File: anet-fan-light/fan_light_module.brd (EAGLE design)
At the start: 10 parts, among them X1 12V, X2 EXT-FAN, X3 Z-PROBE, X4 ANET-Z-INPUT

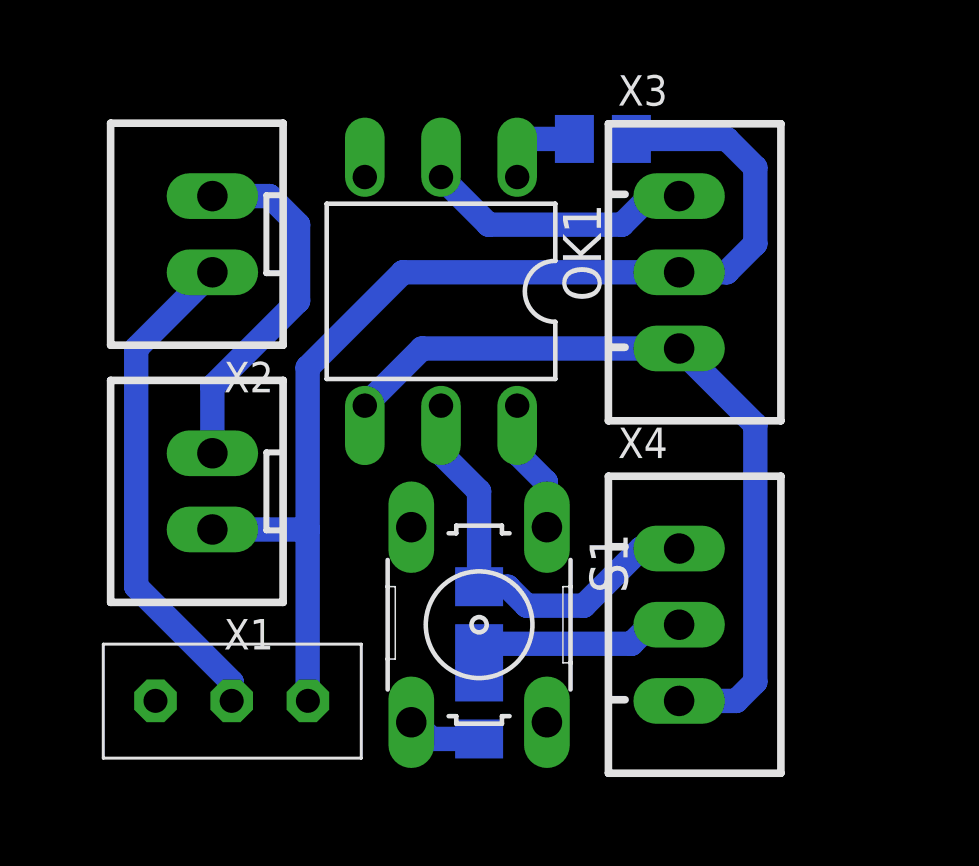
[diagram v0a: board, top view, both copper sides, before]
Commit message: new projects
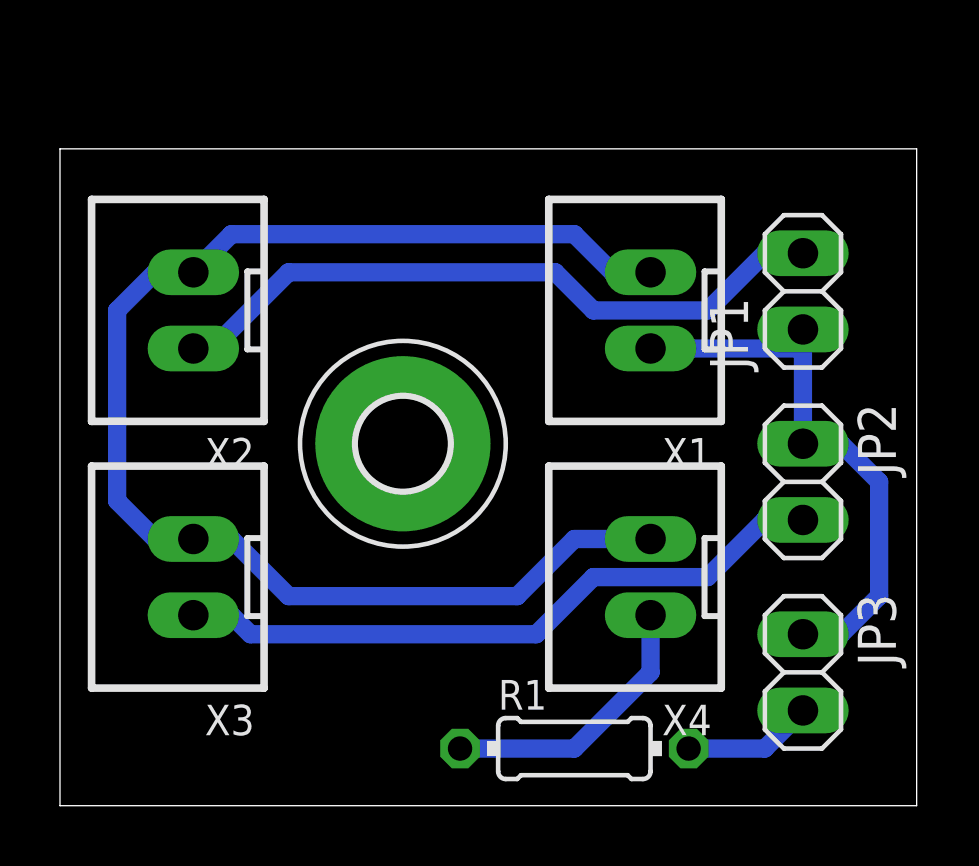
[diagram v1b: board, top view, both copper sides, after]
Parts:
- removed OK1: CNY17, optocoupler:DIL06
- removed R2: 10k, rcl:M0805
- removed R3: (no value), rcl:M0805
- removed S1: (no value), switch-omron:B3F-10XX
- removed S2: (no value), _MY_OWN_LIB:THIN
- added H1: MOUNT-PAD-ROUND3.0, holes:3,0-PAD
- added JP1, JP2, JP3: (no value), pinhead:1X02
- R1: value 10k -> (none); device rcl:M0805 -> rcl:0204/7
- X1: value 12V -> IN-12V
- X2: value EXT-FAN -> NOZ-FAN
- X3: value Z-PROBE -> LIGHT; device Rembrandt Electronics - JST XH Connectors v1-0:JST-XH-03-PACKAGE-LONG-PAD -> Rembrandt Electronics - JST XH Connectors v1-0:JST-XH-02-PACKAGE-LONG-PAD
- X4: value ANET-Z-INPUT -> EXT-FAN; device Rembrandt Electronics - JST XH Connectors v1-0:JST-XH-03-PACKAGE-LONG-PAD -> Rembrandt Electronics - JST XH Connectors v1-0:JST-XH-02-PACKAGE-LONG-PAD
- moved X3 19.1 mm to (4.45, 7.62), turned to 90 degrees
- moved X1 15.8 mm to (19.7, 16.5)
- moved R1 5.46 mm to (17.1, 1.91), flipped to the top, turned to 0 degrees
- moved X2 2.62 mm to (4.45, 16.5)
- moved X4 1.85 mm to (19.7, 7.62), turned to 90 degrees
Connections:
- removed net +5V: R1.2, R2.2, X4.2
- removed net N$5: OK1.6, S1.1, S1.2
- removed net N$6: OK1.1, R3.1
- removed net N$7: OK1.2, X3.1
- new net N$3: R1.1, X4.1
- net +12V: now also JP1.1, JP2.1, JP3.1; no longer R3.2, S2.P$1, X3.2
- net GND: now also X3.2, X4.2; no longer OK1.4, X3.3, X4.3
- net N$1: now also JP1.2; no longer S2.P$2
- net N$2: now also JP2.2, X3.1; no longer OK1.5, R1.1, X4.1
- net N$4: now also JP3.2, R1.2; no longer R2.1, S1.3, S1.4
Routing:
- net +12V: track 38.0 -> 18.8 mm
- net N$3: track 0.00 -> 9.31 mm
- net N$7: track 8.99 -> 0.00 mm
- net N$2: track 14.3 -> 22.2 mm
- net GND: track 38.3 -> 45.6 mm
- net +5V: track 7.25 -> 0.00 mm
- net N$1: track 16.7 -> 22.7 mm
- net N$5: track 4.46 -> 0.00 mm
- net N$6: track 3.18 -> 0.00 mm
- net N$4: track 2.48 -> 4.34 mm
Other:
- board outline added: 28.6 x 21.9 mm
